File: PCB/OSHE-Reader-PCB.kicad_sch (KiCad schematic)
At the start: 1 part, among them U1 ESP32-S3-WROOM-1-N8R8

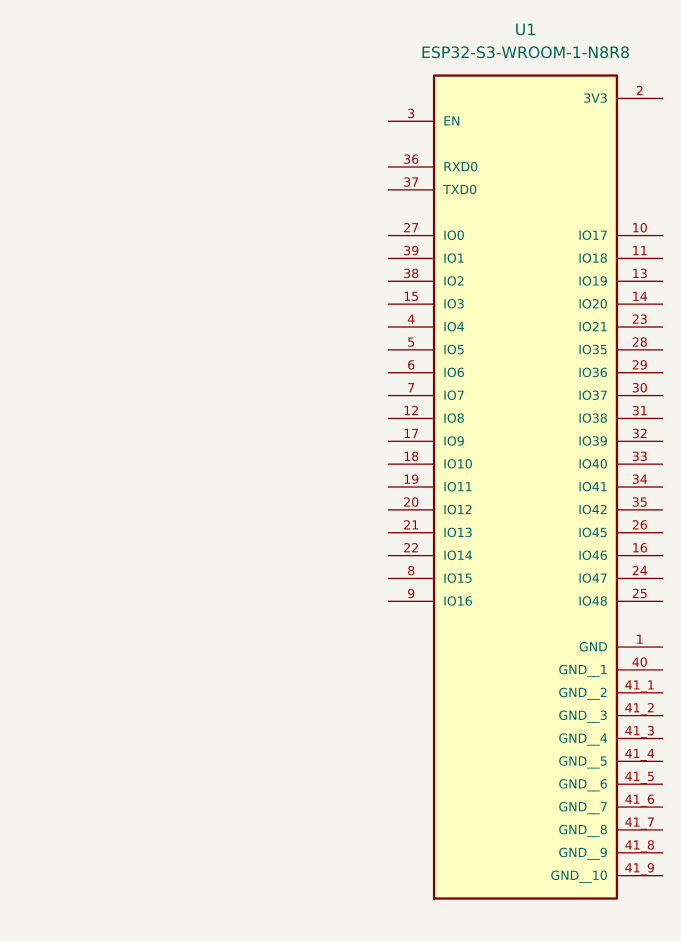
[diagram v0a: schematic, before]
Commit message: Actually working now I think
Got new footprints working mainly for the esp
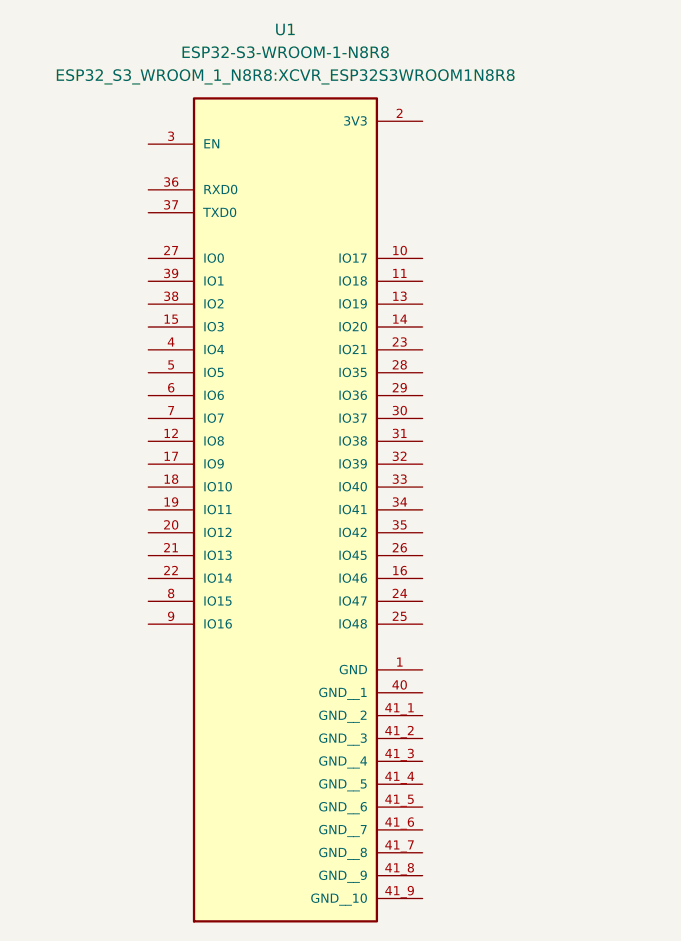
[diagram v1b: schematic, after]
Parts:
- U1: footprint ESP32-S3-WROOM-1-N8R8:XCVR_ESP32S3WROOM1N8R8 -> ESP32_S3_WROOM_1_N8R8:XCVR_ESP32S3WROOM1N8R8; AVAILABILITY In Stock -> (none); PRICE None -> (none); PURCHASE-URL https://pricing.snapeda.com/search/part/ESP32S3WROOM1N8R8/?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 -> (none)
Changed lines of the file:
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@@
 	(symbol
 		(lib_id "ESP32-S3-WROOM-1-N8R8:ESP32-S3-WROOM-1-N8R8")
-		(at 86.36 59.69 0)
+		(at 59.69 62.23 0)
 		(unit 1)
 		(body_style 1)
@@
 		(fields_autoplaced yes)
 		(property "Reference" "U1"
-			(at 86.36 21.59 0)
+			(at 59.69 21.59 0)
 			(show_name no)
 			(do_not_autoplace no)
@@
 		)
 		(property "Value" "ESP32-S3-WROOM-1-N8R8"
-			(at 86.36 24.13 0)
-			(show_name no)
-			(do_not_autoplace no)
-			(effects
-				(font
-					(size 1.27 1.27)
-				)
-			)
-		)
-		(property "Footprint" "ESP32-S3-WROOM-1-N8R8:XCVR_ESP32S3WROOM1N8R8"
-			(at 86.36 59.69 0)
-			(hide yes)
-			(show_name no)
-			(do_not_autoplace no)
-			(effects
-				(font
-					(size 1.27 1.27)
-				)
-				(justify bottom)
+			(at 59.69 24.13 0)
+			(show_name no)
+			(do_not_autoplace no)
+			(effects
+				(font
+					(size 1.27 1.27)
+				)
+			)
+		)
+		(property "Footprint" "ESP32_S3_WROOM_1_N8R8:XCVR_ESP32S3WROOM1N8R8"
+			(at 59.69 26.67 0)
+			(show_name no)
+			(do_not_autoplace no)
+			(effects
+				(font
+					(size 1.27 1.27)
+				)
 			)
 		)
 		(property "Datasheet" ""
-			(at 86.36 59.69 0)
+			(at 59.69 62.23 0)
 			(hide yes)
 			(show_name no)
@@
 		)
 		(property "Description" "Bluetooth, WiFi 802.11b/g/n, Bluetooth v5.0 Transceiver Module 2.4GHz PCB Trace Surface Mount"
-			(at 86.36 59.69 0)
+			(at 59.69 62.23 0)
 			(hide yes)
 			(show_name no)
@@
 		)
 		(property "MF" "Espressif Systems"
-			(at 86.36 59.69 0)
+			(at 59.69 62.23 0)
 			(hide yes)
 			(show_name no)
@@
 		)
 		(property "PACKAGE" "SMD-41 Espressif Systems"
-			(at 86.36 59.69 0)
-			(hide yes)
-			(show_name no)
-			(do_not_autoplace no)
-			(effects
-				(font
-					(size 1.27 1.27)
-				)
-				(justify bottom)
-			)
-		)
-		(property "PRICE" "None"
-			(at 86.36 59.69 0)
+			(at 59.69 62.23 0)
+			(hide yes)
+			(show_name no)
+			(do_not_autoplace no)
+			(effects
+				(font
+					(size 1.27 1.27)
+				)
+				(justify bottom)
+			)
+		)
+		(property "PRICE" ""
+			(at 59.69 62.23 0)
 			(hide yes)
 			(show_name no)
@@
 		)
 		(property "MP" "ESP32S3WROOM1N8R8"
-			(at 86.36 59.69 0)
-			(hide yes)
-			(show_name no)
-			(do_not_autoplace no)
-			(effects
-				(font
-					(size 1.27 1.27)
-				)
-				(justify bottom)
-			)
-		)
-		(property "AVAILABILITY" "In Stock"
-			(at 86.36 59.69 0)
-			(hide yes)
-			(show_name no)
-			(do_not_autoplace no)
-			(effects
-				(font
-					(size 1.27 1.27)
-				)
-				(justify bottom)
-			)
-		)
-		(property "PURCHASE-URL" "https://pricing.snapeda.com/search/part/ESP32S3WROOM1N8R8/?ref=eda"
-			(at 86.36 59.69 0)
-			(hide yes)
-			(show_name no)
-			(do_not_autoplace no)
-			(effects
-				(font
-					(size 1.27 1.27)
-				)
-				(justify bottom)
-			)
+			(at 59.69 62.23 0)
+			(hide yes)
+			(show_name no)
+			(do_not_autoplace no)
+			(effects
+				(font
+					(size 1.27 1.27)
+				)
+				(justify bottom)
+			)
+		)
+		(property "AVAILABILITY" ""
+			(at 59.69 62.23 0)
+			(hide yes)
+			(show_name no)
+			(do_not_autoplace no)
+			(effects
+				(font
+					(size 1.27 1.27)
+				)
+				(justify bottom)
+			)
+		)
+		(property "PURCHASE-URL" ""
+			(at 59.69 62.23 0)
+			(hide yes)
+			(show_name no)
+			(do_not_autoplace no)
+			(effects
+				(font
+					(size 1.27 1.27)
+				)
+				(justify bottom)
+			)
+		)
+		(pin "6"
+		)
+		(pin "8"
+		)
+		(pin "7"
+		)
+		(pin "5"
+		)
+		(pin "9"
+		)
+		(pin "14"
+		)
+		(pin "10"
+		)
+		(pin "12"
+		)
+		(pin "11"
+		)
+		(pin "13"
+		)
+		(pin "19"
+		)
+		(pin "16"
+		)
+		(pin "17"
+		)
+		(pin "18"
+		)
+		(pin "15"
+		)
+		(pin "3"
 		)
 		(pin "2"
 		)
-		(pin "5"
-		)
-		(pin "9"
-		)
-		(pin "11"
-		)
-		(pin "8"
-		)
-		(pin "19"
-		)
-		(pin "7"
-		)
-		(pin "14"
-		)
-		(pin "13"
-		)
-		(pin "16"
-		)
-		(pin "6"
-		)
-		(pin "3"
-		)
 		(pin "1"
 		)
-		(pin "18"
-		)
-		(pin "12"
-		)
-		(pin "17"
-		)
-		(pin "15"
-		)
 		(pin "4"
 		)
-		(pin "10"
+		(pin "41_6"
+		)
+		(pin "41_3"
+		)
+		(pin "41_4"
+		)
+		(pin "24"
+		)
+		(pin "41_7"
+		)
+		(pin "28"
 		)
 		(pin "23"
 		)
+		(pin "27"
+		)
+		(pin "41_5"
+		)
+		(pin "39"
+		)
+		(pin "41_8"
+		)
+		(pin "26"
+		)
+		(pin "35"
+		)
+		(pin "22"
+		)
+		(pin "34"
+		)
+		(pin "31"
+		)
+		(pin "25"
+		)
+		(pin "37"
+		)
+		(pin "40"
+		)
+		(pin "30"
+		)
+		(pin "21"
+		)
+		(pin "33"
+		)
+		(pin "38"
+		)
+		(pin "36"
+		)
+		(pin "20"
+		)
+		(pin "29"
+		)
+		(pin "41_2"
+		)
+		(pin "41_1"
+		)
 		(pin "32"
 		)
-		(pin "41_5"
-		)
-		(pin "41_1"
-		)
-		(pin "41_2"
-		)
-		(pin "41_6"
-		)
-		(pin "35"
-		)
-		(pin "25"
-		)
-		(pin "41_8"
-		)
-		(pin "41_7"
-		)
-		(pin "37"
-		)
-		(pin "34"
-		)
-		(pin "27"
-		)
-		(pin "30"
-		)
-		(pin "33"
-		)
-		(pin "39"
-		)
-		(pin "22"
-		)
-		(pin "40"
-		)
-		(pin "41_3"
-		)
-		(pin "21"
-		)
-		(pin "24"
-		)
-		(pin "28"
-		)
-		(pin "31"
-		)
-		(pin "41_4"
-		)
-		(pin "36"
-		)
-		(pin "20"
-		)
-		(pin "38"
-		)
-		(pin "26"
-		)
-		(pin "29"
-		)
 		(pin "41_9"
